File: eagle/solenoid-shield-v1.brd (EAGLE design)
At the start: 49.2 x 53.3 mm, 13 parts, among them Q1 ARDUINOR3-NOIOREF-NOTEXT, SW1 SPST_TACT-EVQQ2, SW2 SPST_TACT-EVQQ2

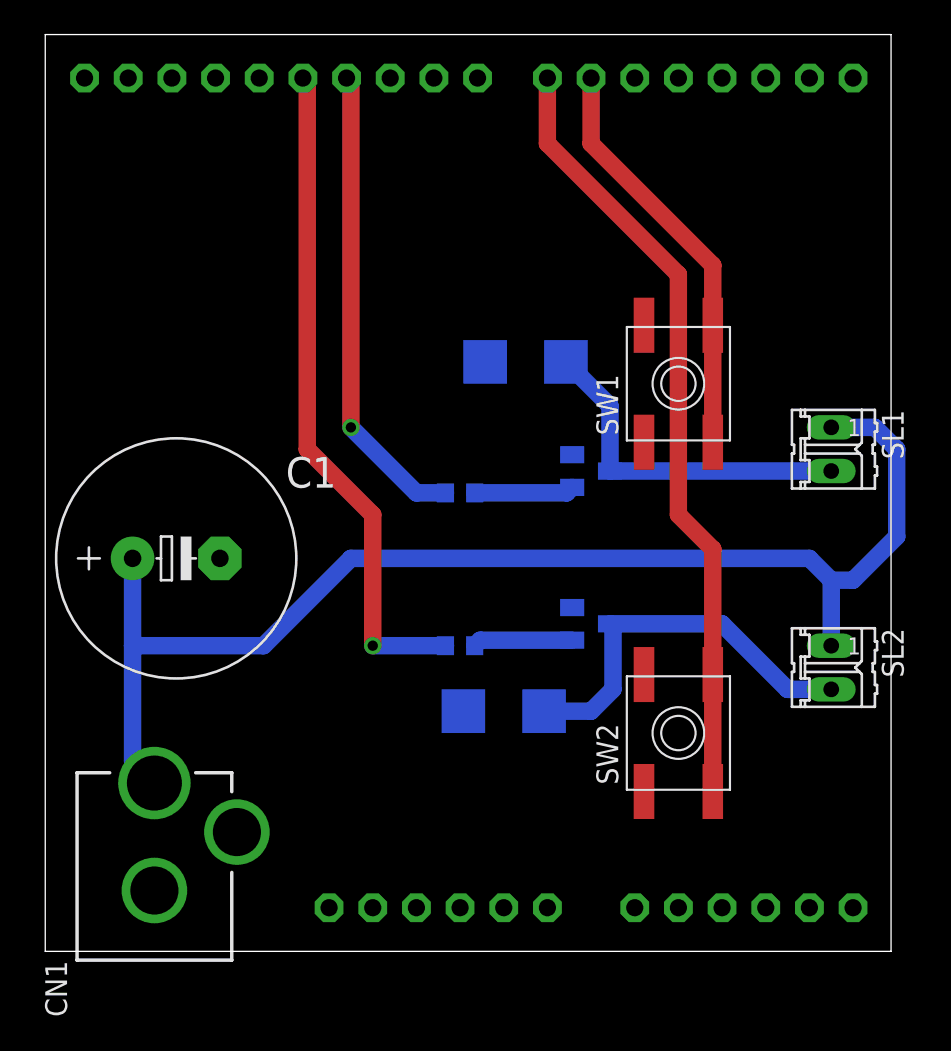
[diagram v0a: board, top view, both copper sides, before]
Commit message: Finished v1 of the shield
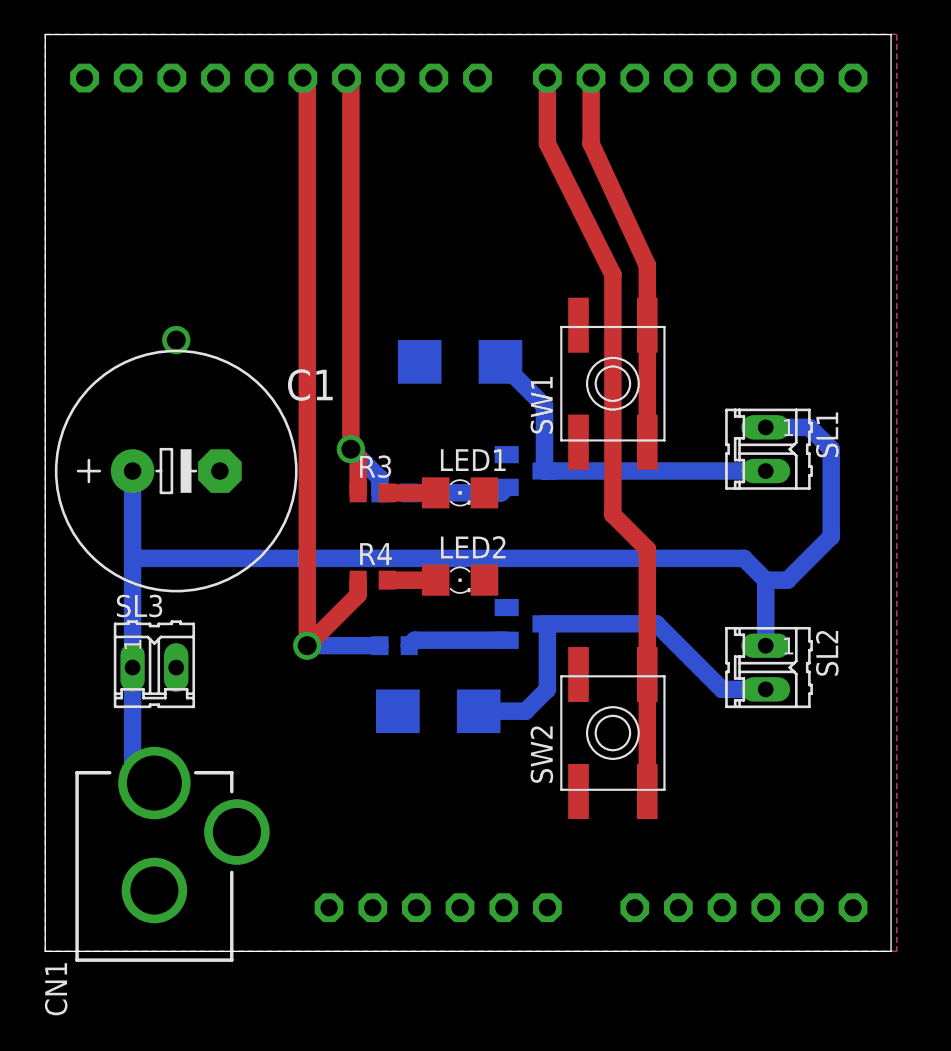
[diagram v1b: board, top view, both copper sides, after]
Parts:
- added LED1, LED2: (no value), adafruit:1206
- added R3: 3k3, adafruit:R0603
- added R4: 1k, adafruit:R0603
- added SL3: (no value), con-amp-quick:02P
- moved C1 5.08 mm to (7.62, 27.9)
- moved D1 3.81 mm to (24.1, 34.3)
- moved D2 3.81 mm to (22.9, 14.0)
- moved SL1 3.81 mm to (41.9, 29.2)
- moved SL2 3.81 mm to (41.9, 16.5)
- moved R1 3.81 mm to (20.3, 26.7)
- moved R2 3.81 mm to (20.3, 17.8)
- moved T1 3.81 mm to (27.9, 27.9)
- moved T2 3.81 mm to (27.9, 19.1)
- moved SW1 3.81 mm to (33.0, 33.0)
- moved SW2 3.81 mm to (33.0, 12.7)
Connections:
- new net N$1: LED2.A, R4.2
- new net N$4: LED1.A, R3.2
- net +12V: now also SL3.1
- net D11: now also R3.1
- net D12: now also R4.1
- net GND: now also LED2.C, SL3.2
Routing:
- net D12: track 38.9 -> 42.4 mm
- net N$4: track 0.00 -> 2.81 mm
- net N$1: track 0.00 -> 2.81 mm
- net D7: track 45.5 -> 43.2 mm
- net D6: track 24.1 -> 21.9 mm
- net +12V: track 75.0 -> 74.1 mm
- added copper zone on layer 1, net GND
- added copper zone on layer 16, net GND
